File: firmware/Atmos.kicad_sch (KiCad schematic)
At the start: 56 parts, among them J1 AS3935 breakout, J2 BME280 breakout, J3 USB_C_Receptacle_USB2.0_16P, J4 Micro_SD_Card, J5 Solar power input, J6 Conn_Coaxial, Q1 PMOS_Substrate, Q2 PMOS_Substrate, Q3 PMOS_Substrate, SW2 SW_Push, U1 ESP32-S3-WROOM-1, U10 TPS22918DBVR, U11 MAX17048G_T10, U12 CN3791, U13 SGP40-D-R4, U2 AP2112K-3.3, U3 DS3231M, U4 PMS5003, U5 LTC4412xS6, U7 RFM95W-915S2, U8 USBLC6-2SC6, U9 TPS61023DRLR

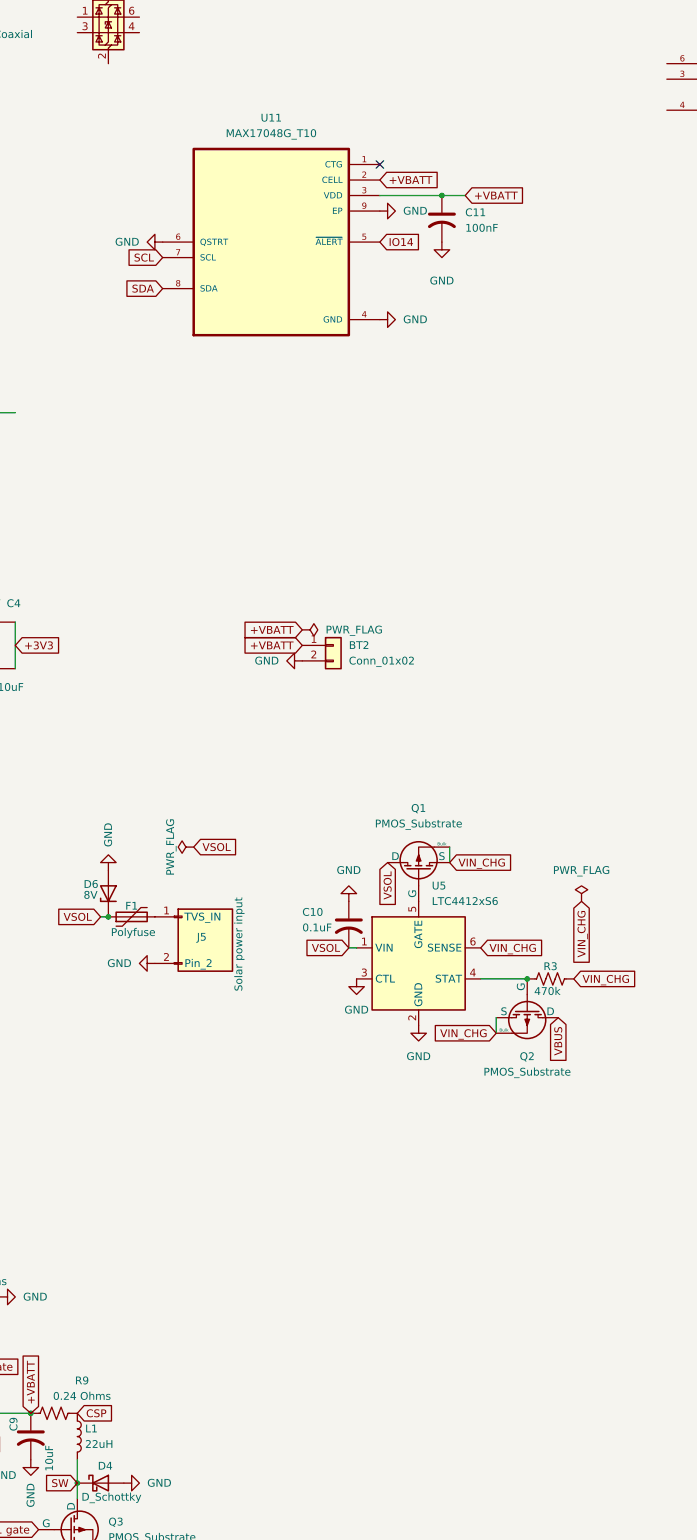
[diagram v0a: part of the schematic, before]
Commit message: U11 touchup
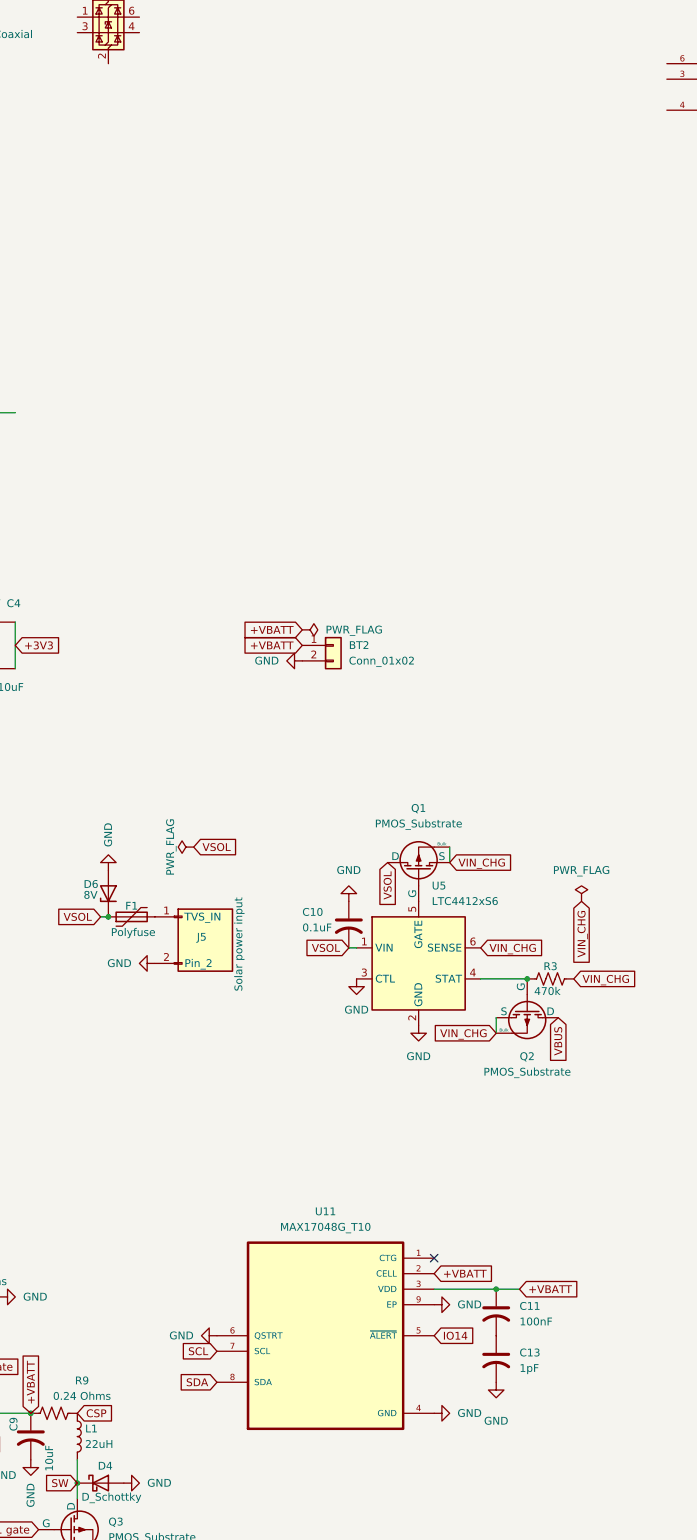
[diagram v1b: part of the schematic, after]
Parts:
- added C13: 1pF, symbol Device:C_US
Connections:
- net GND: now also C13.2; no longer C11.2
- new net: C11.2, C13.1
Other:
- moved on the sheet: C11, U11

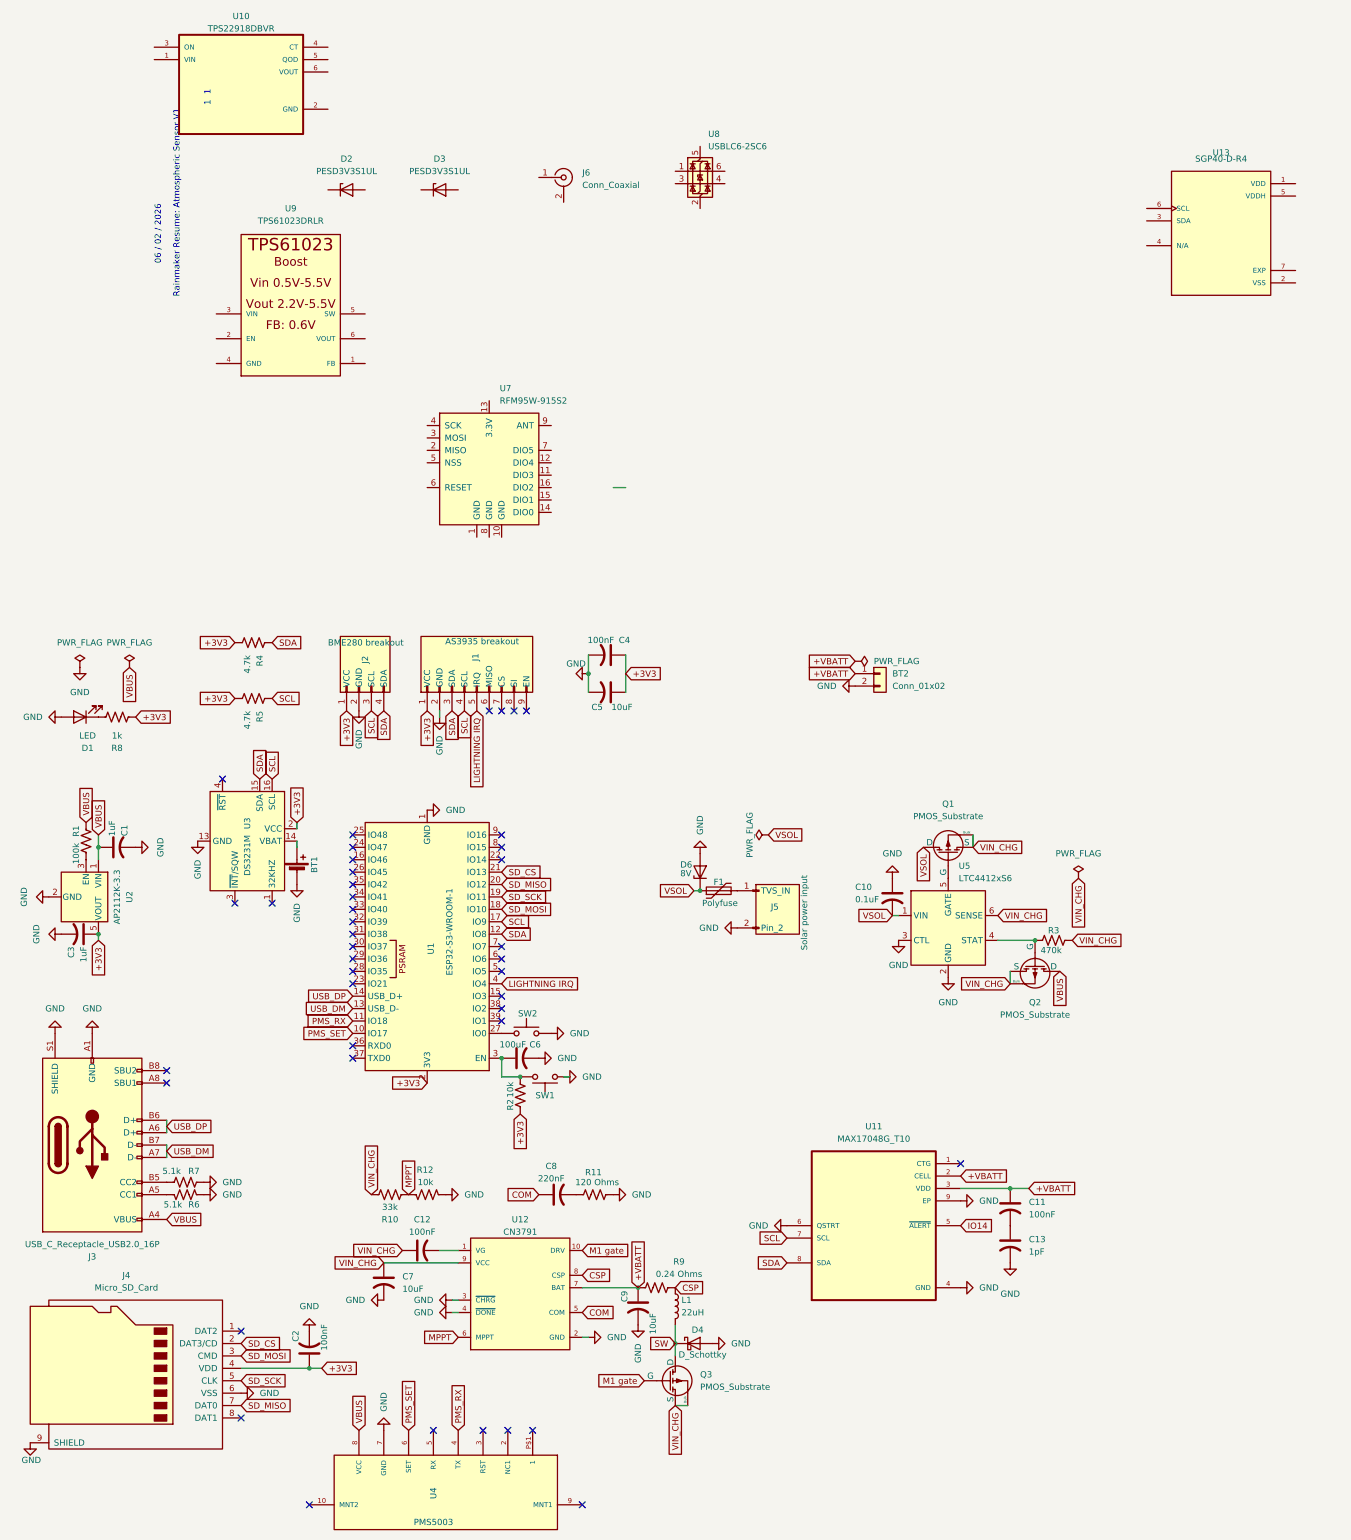
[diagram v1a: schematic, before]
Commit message: TPS init
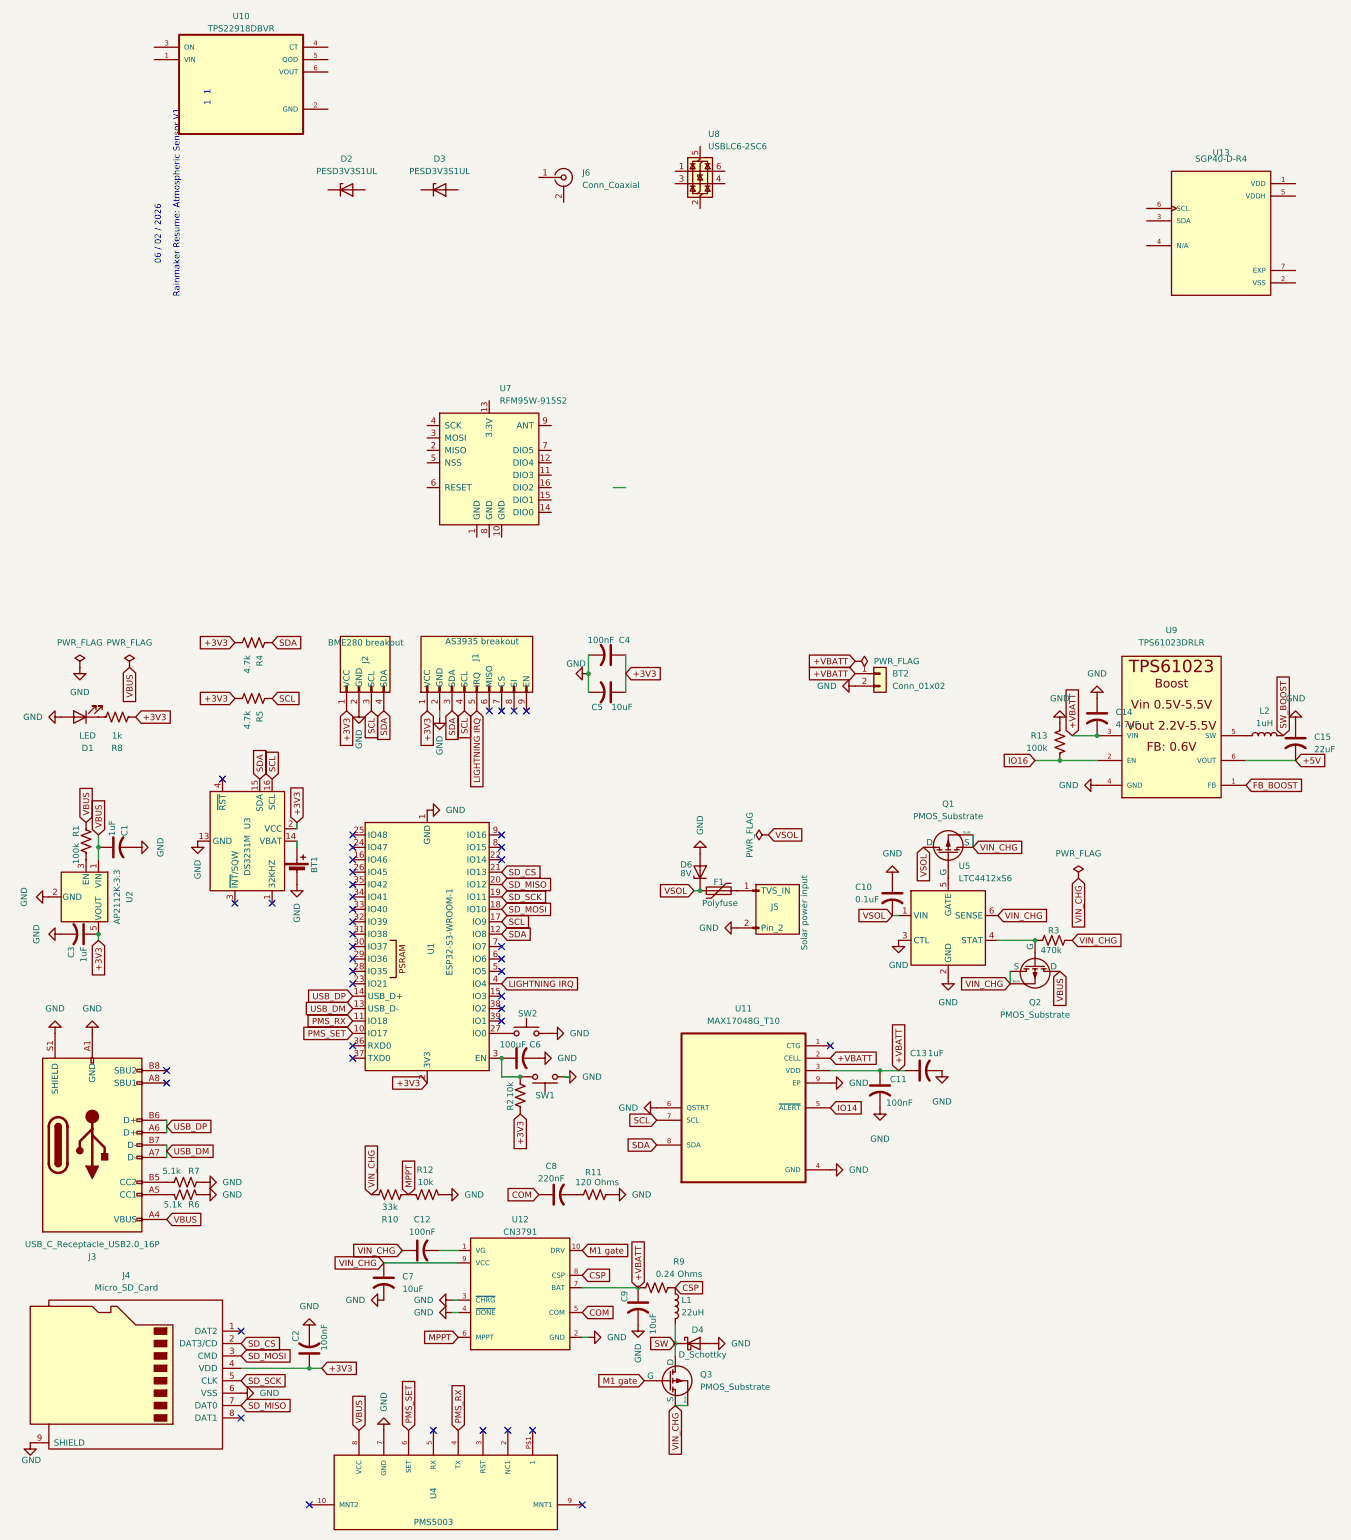
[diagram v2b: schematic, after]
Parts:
- added C14: 4.7uF, symbol Device:C_US
- added C15: 22uF, symbol Device:C_US
- added L2: 1uH, symbol Device:L
- added R13: 100k, symbol Device:R_US
- C13: value 1pF -> 1uF
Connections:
- net +VBATT: now also C13.1, U9.3 (VIN), C14.2
- net GND: now also C11.2, U9.4 (GND), C14.1, C15.1, R13.1
- net FB_BOOST: now reaches U9.1 (FB)
- net IO16: now reaches U9.2 (EN)
- net IO16: now also R13.2
- net at U9.5 (SW): now also L2.1
- net +5V: now reaches U9.6 (VOUT)
- net +5V: now also C15.2
- new net SW_BOOST: L2.2
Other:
- moved on the sheet: C11, C13, U11, U9
